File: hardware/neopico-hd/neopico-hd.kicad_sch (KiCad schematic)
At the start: 1 part

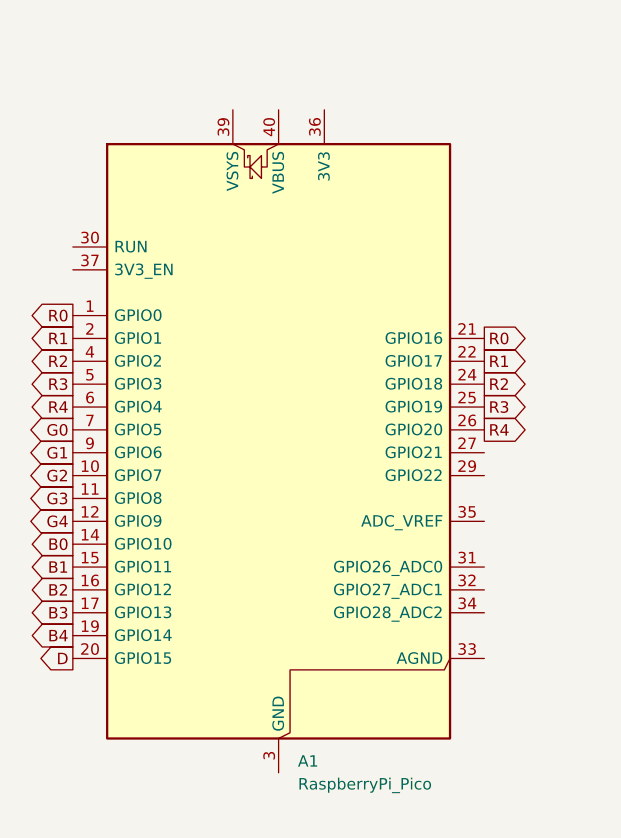
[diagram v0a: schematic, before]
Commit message: Update sch
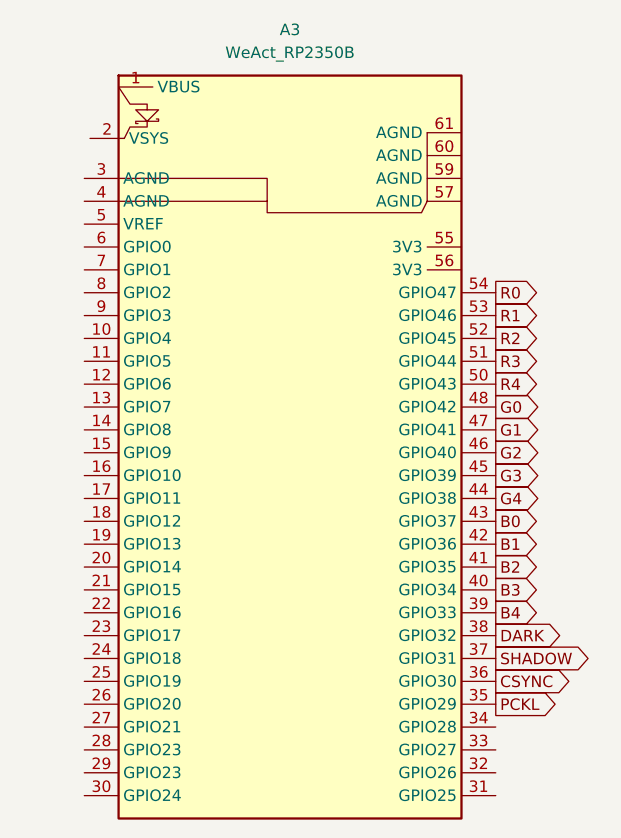
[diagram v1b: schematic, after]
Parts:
- removed A1: RaspberryPi_Pico, Module:RaspberryPi_Pico_Common_Unspecified, symbol MCU_Module:RaspberryPi_Pico
- added A3: WeAct_RP2350B, symbol Dudu:WeAct_RP2350B
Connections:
- net B0: now also A3.43 (GPIO37)
- net B1: now also A3.42 (GPIO36)
- net B2: now also A3.41 (GPIO35)
- net B3: now also A3.40 (GPIO34)
- net B4: now also A3.39 (GPIO33)
- net G0: now also A3.48 (GPIO42)
- net G1: now also A3.47 (GPIO41)
- net G2: now also A3.46 (GPIO40)
- net G3: now also A3.45 (GPIO39)
- net G4: now also A3.44 (GPIO38)
- net R0: now also A3.54 (GPIO47)
- net R1: now also A3.53 (GPIO46)
- net R2: now also A3.52 (GPIO45)
- net R3: now also A3.51 (GPIO44)
- net R4: now also A3.50 (GPIO43)
- new net CSYNC: A3.36 (GPIO30)
- new net DARK: A3.38 (GPIO32)
- new net PCKL: A3.35 (GPIO29)
- new net SHADOW: A3.37 (GPIO31)
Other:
- company: (none) -> https://www.github.com/fliperama86/neopico-hd
- title: (none) -> NeoPico HD
